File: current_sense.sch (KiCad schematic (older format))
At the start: 2 parts, among them U1 ACS712xLCTR-30A

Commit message: started layout
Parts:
- C1: symbol open-automation:C_10nF -> dimmer-2ch-rescue:C_10nF-open-automation
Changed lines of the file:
@@
 EESchema Schematic File Version 4
-EELAYER 29 0
+LIBS:dimmer-2ch-cache
+EELAYER 26 0
 EELAYER END
 $Descr A4 11693 8268
 encoding utf-8
-Sheet 5 6
+Sheet 2 6
 Title ""
 Date ""
@@
 	5725 2800 5725 2750
 $Comp
-L open-automation:C_10nF C?
+L dimmer-2ch-rescue:C_10nF-open-automation C?
 U 1 1 5BF2198C
 P 6175 2650

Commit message: finished layout, final check
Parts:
- U1: symbol Sensor_Current:ACS712xLCTR-30A -> dimmer-2ch-rescue:ACS712xLCTR-30A-Sensor_Current
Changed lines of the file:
@@
 $EndDescr
 $Comp
-L Sensor_Current:ACS712xLCTR-30A U?
+L dimmer-2ch-rescue:ACS712xLCTR-30A-Sensor_Current U?
 U 1 1 5BF208D1
 P 5725 2350
@@
 $EndComp
 $Comp
-L power:GND #PWR?
+L dimmer-2ch-rescue:GND-power #PWR?
 U 1 1 5BF2121D
 P 5725 2800
@@
 	6175 2450 6175 2500
 $Comp
-L power:GND #PWR?
+L dimmer-2ch-rescue:GND-power #PWR?
 U 1 1 5BF22381
 P 6175 2850

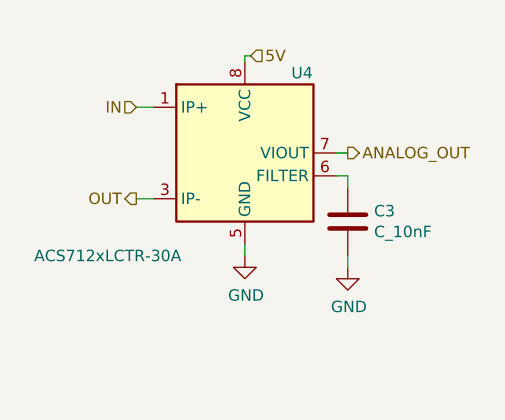
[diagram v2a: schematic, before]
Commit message: ready for board house
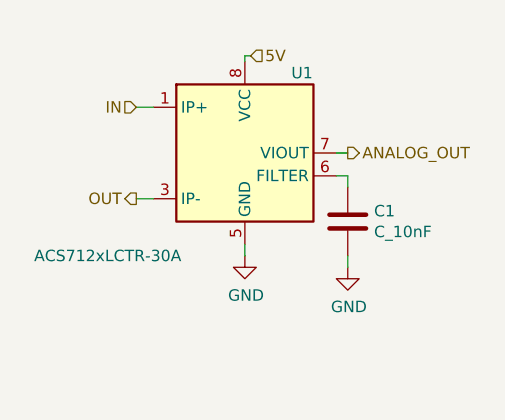
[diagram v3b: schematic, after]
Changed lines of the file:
@@
 AR Path="/5BF2BC14/5BF208D1" Ref="U1"  Part="1"
 AR Path="/5BF337E0/5BF208D1" Ref="U4"  Part="1"
-F 0 "U4" H 5975 2700 50  0000 C CNN
+F 0 "U1" H 5975 2700 50  0000 C CNN
 F 1 "ACS712xLCTR-30A" H 5125 1900 50  0000 C CNN
 F 2 "Package_SO:SOIC-8_3.9x4.9mm_P1.27mm" H 5825 2000 50  0001 L CIN
@@
 AR Path="/5BF2BC14/5BF2198C" Ref="C1"  Part="1"
 AR Path="/5BF337E0/5BF2198C" Ref="C3"  Part="1"
-F 0 "C3" H 6290 2696 50  0000 L CNN
+F 0 "C1" H 6290 2696 50  0000 L CNN
 F 1 "C_10nF" H 6290 2605 50  0000 L CNN
 F 2 "Capacitor_SMD:C_0603_1608Metric_Pad1.05x0.95mm_HandSolder" H 6275 2950 50  0001 C CNN
